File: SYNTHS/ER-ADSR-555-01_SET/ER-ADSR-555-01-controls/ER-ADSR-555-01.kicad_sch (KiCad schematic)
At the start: 33 parts, among them J1 Conn_02x05, J2 PJ-301BM, J3 PJ-301BM, Q1 2N3904, Q2 2N3904, Q3 2N3904, U1 TL072, U2 LM555N

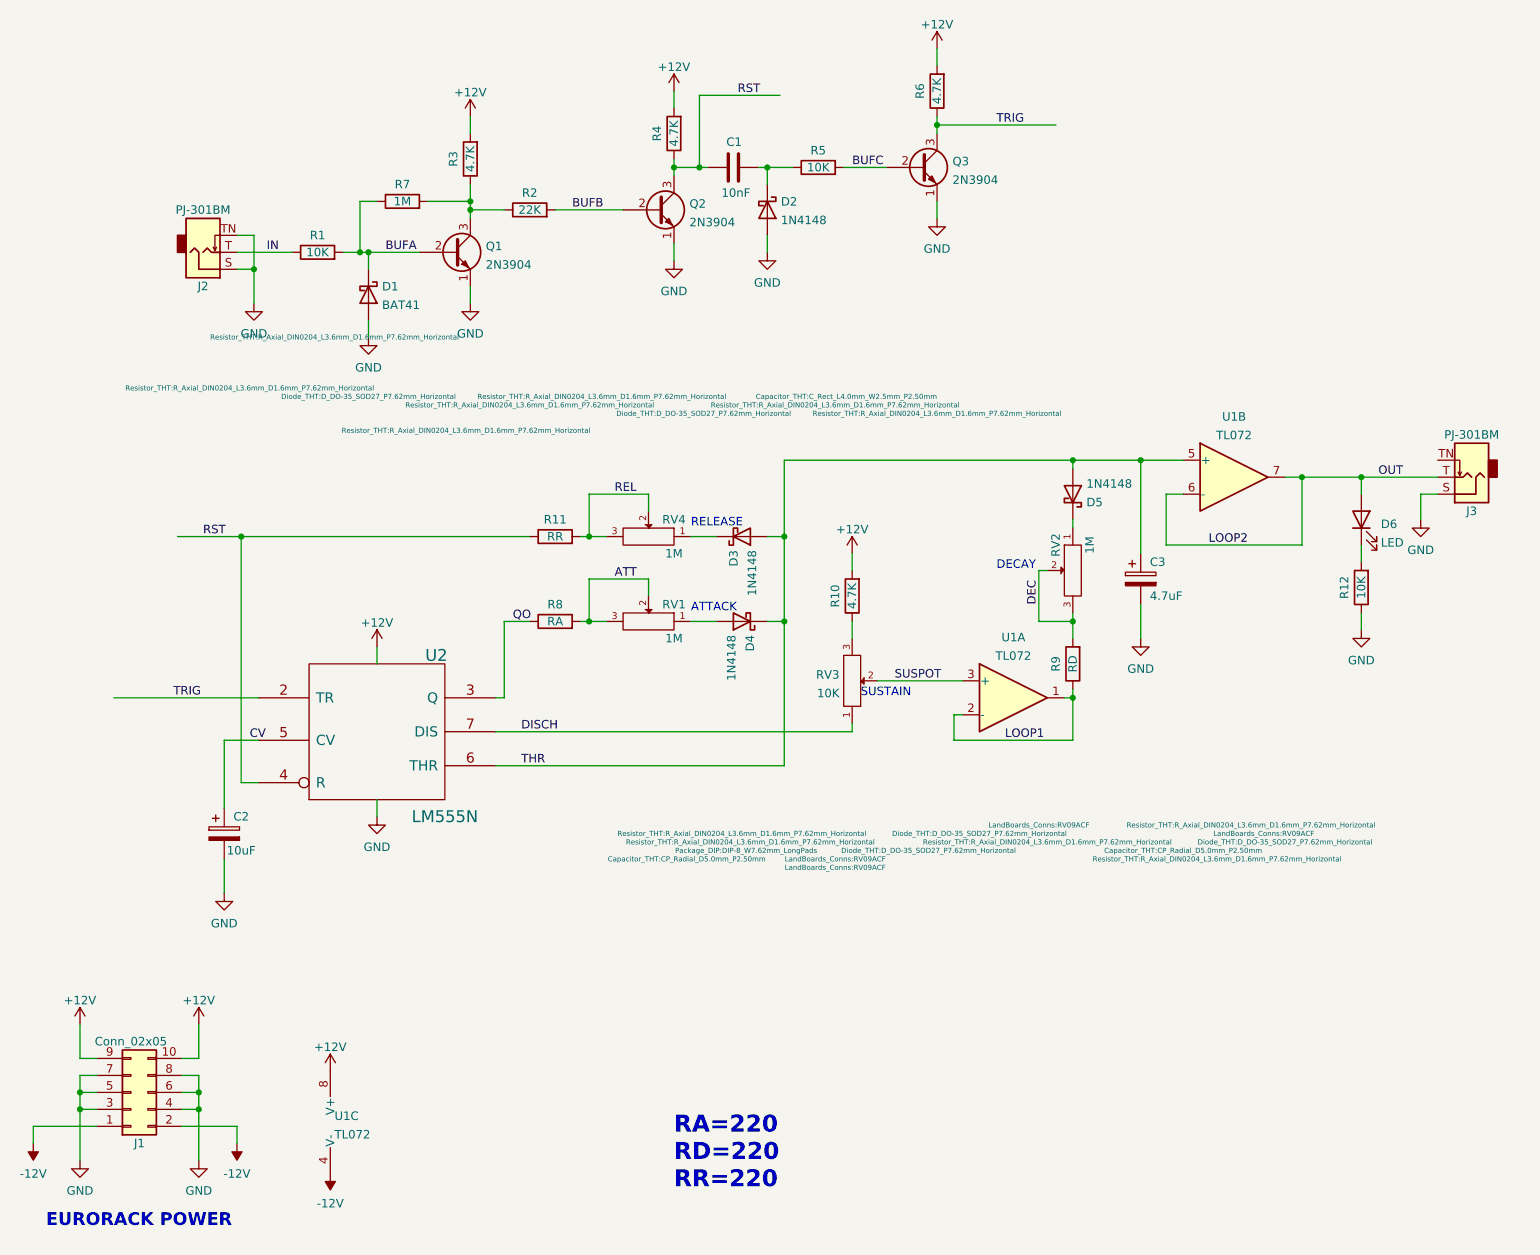
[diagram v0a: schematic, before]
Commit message: ADSR working
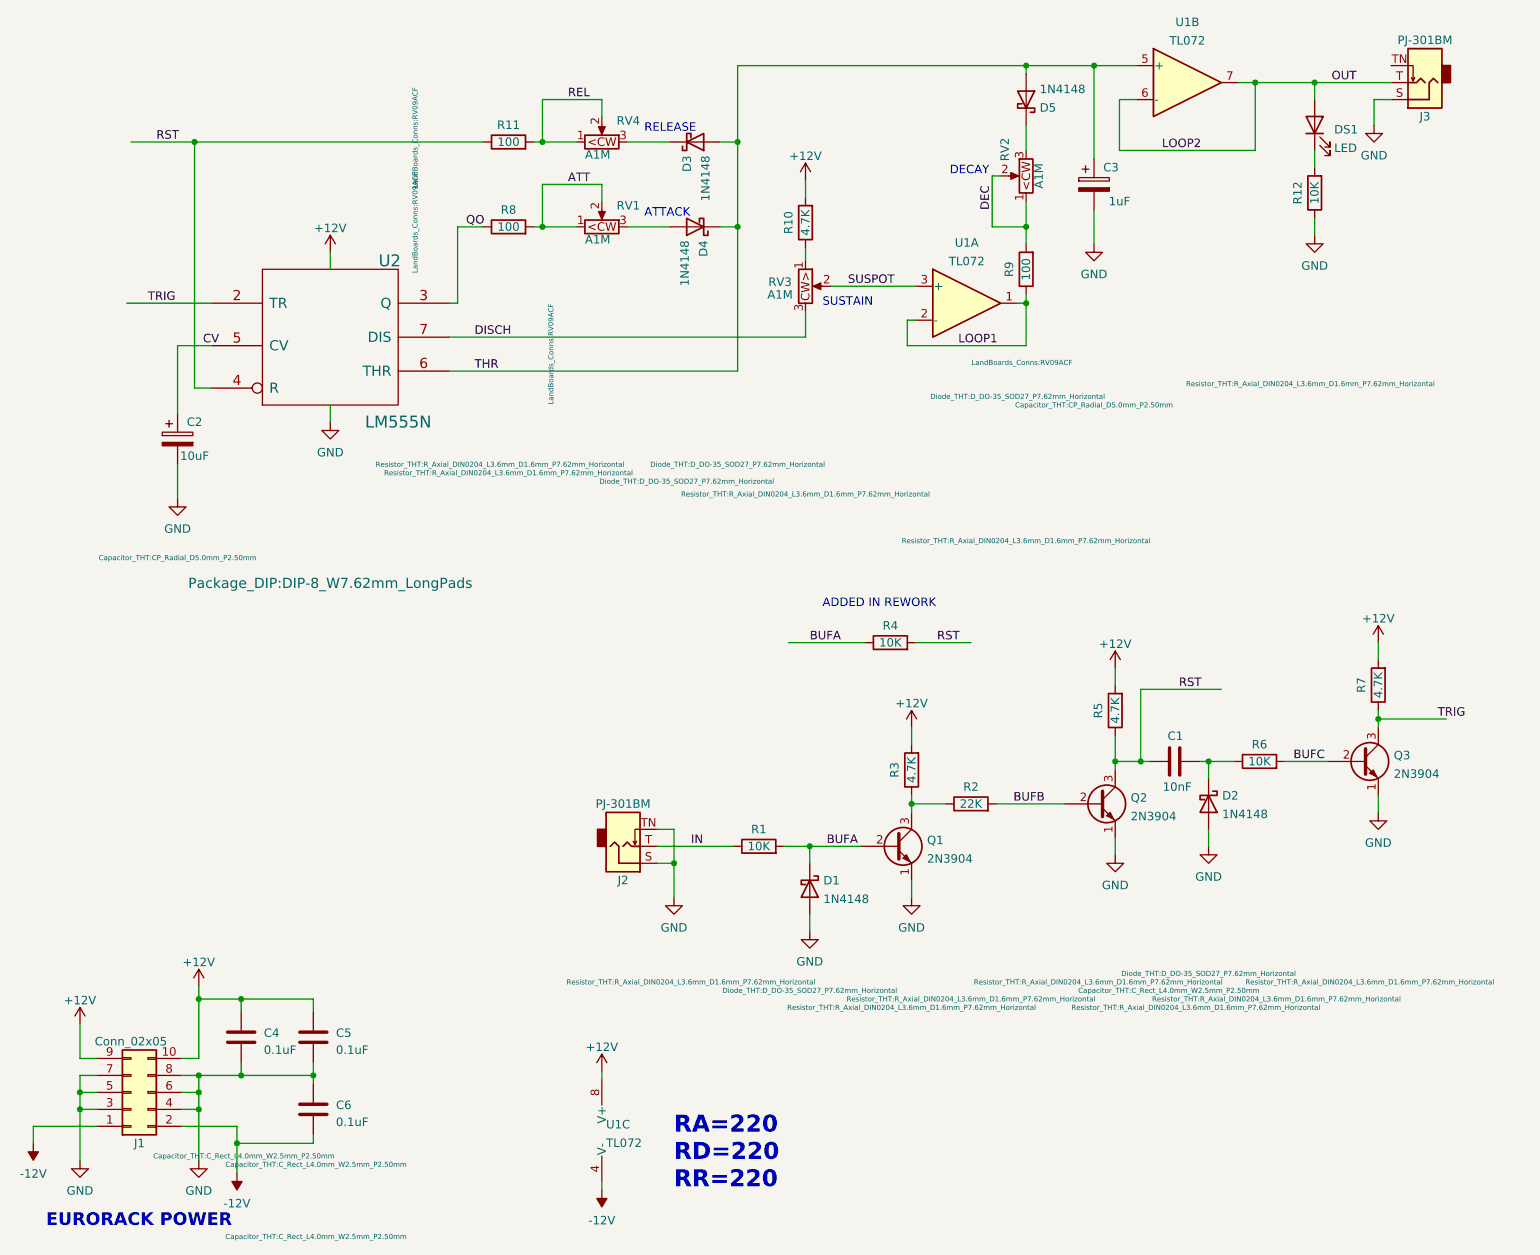
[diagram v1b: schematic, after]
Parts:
- removed R7: 1M, Resistor_THT:R_Axial_DIN0204_L3.6mm_D1.6mm_P7.62mm_Horizontal, symbol Device:R
- removed RV1, RV2, RV4: 1M, LandBoards_Conns:RV09ACF, symbol LandBoards:POT
- removed RV3: 10K, LandBoards_Conns:RV09ACF, symbol LandBoards:POT
- added C4, C5, C6: 0.1uF, Capacitor_THT:C_Rect_L4.0mm_W2.5mm_P2.50mm, symbol Device:C
- added R4: 10K, Resistor_THT:R_Axial_DIN0204_L3.6mm_D1.6mm_P7.62mm_Horizontal, symbol Device:R
- added RV1, RV2, RV4: A1M, LandBoards_Conns:RV09ACF, symbol LandBoards_Conns:R_Pot_CW_PIN3UP
- added RV3: A1M, LandBoards_Conns:RV09ACF, symbol LandBoards_Conns:R_Pot_CW
- C3: value 4.7uF -> 1uF
- D1: value BAT41 -> 1N4148
- Q1, Q2, Q3: footprint Package_TO_SOT_THT:TO-92_Inline -> Package_TO_SOT_THT:TO-92_HandSolder
- R11: value RR -> 100
- R8: value RA -> 100
- R9: value RD -> 100
- renumbered D6 to DS1, R4 to R5, R5 to R6, R6 to R7
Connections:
- net +12V: now also C4.2, C5.2
- net -12V: now also C6.1
- net ATT: now also RV1.1, RV1.2
- net BUFA: now also R4.1
- net DEC: now also RV2.1, RV2.2
- net DISCH: now also RV3.3
- net GND: now also C4.1, C5.1, C6.2
- net REL: now also RV4.1, RV4.2
- net RST: now also R4.2
- net SUSPOT: now also RV3.2
- net at D4.2 (A): now also RV1.3
- net at D5.1 (K): now also RV2.3
- net at D3.1 (K): now also RV4.3
- net at R10.1: now also RV3.1
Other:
- note added: "ADDED IN REWORK"
- title: (none) -> ADSR GENERATOR
- moved on the sheet: C1, C2, C3, D1, D2, D3, D4, D5, DS1, J2, J3, Q1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
